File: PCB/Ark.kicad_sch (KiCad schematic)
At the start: 47 parts, among them P1 mode, P2 down, P3 up, SW1 EC12, SW2 EC12, SW3 EC12, SW4 EC12, SW5 EC12, SW6 EC12, SW7 EC12, SW8 EC12, U1 SeeeduinoXIAO, U2 ATmega328P-P, U3 ATmega328P-P, U4 74HC595

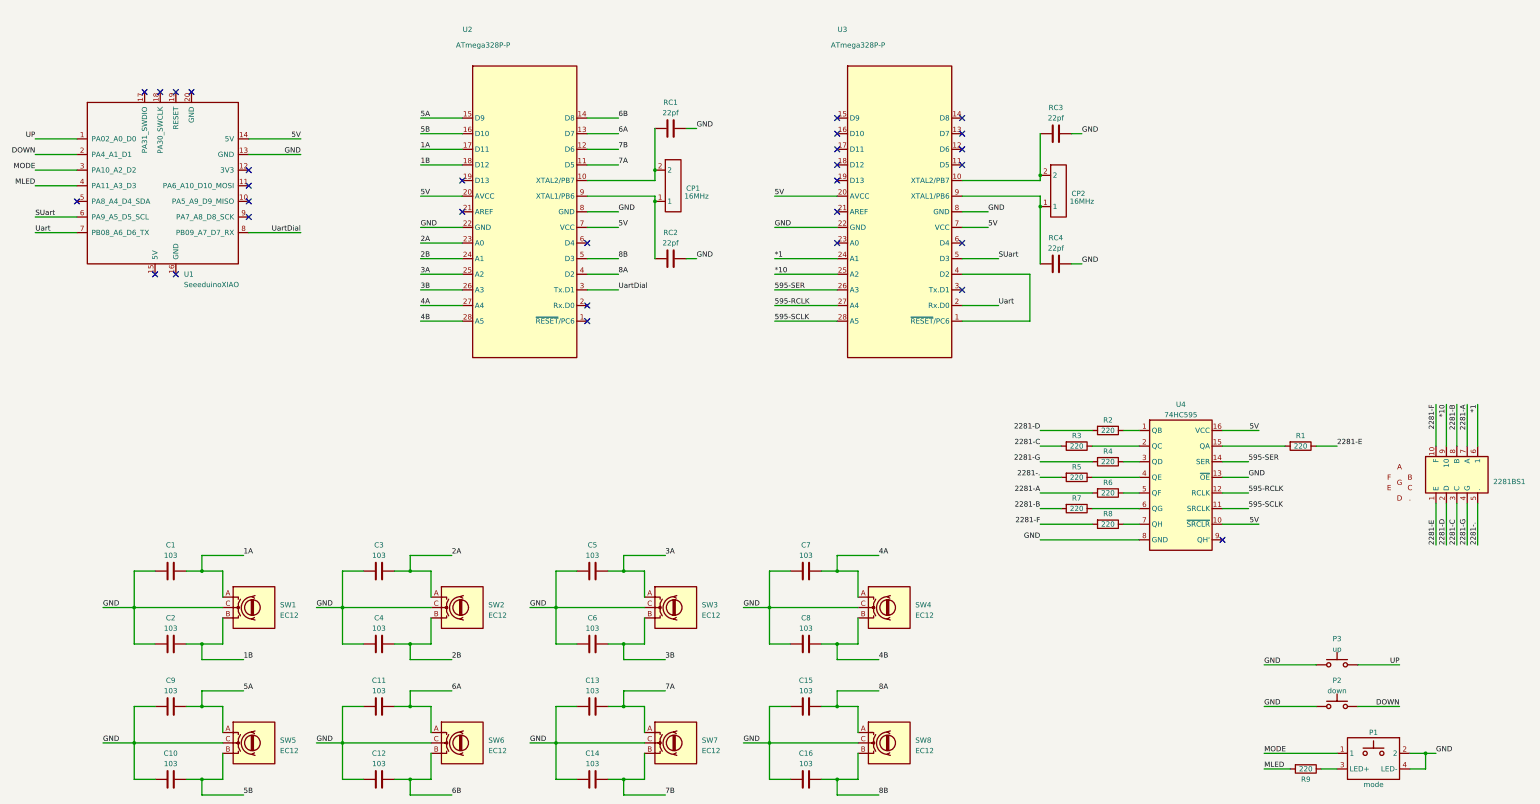
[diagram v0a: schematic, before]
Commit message: Add files via upload
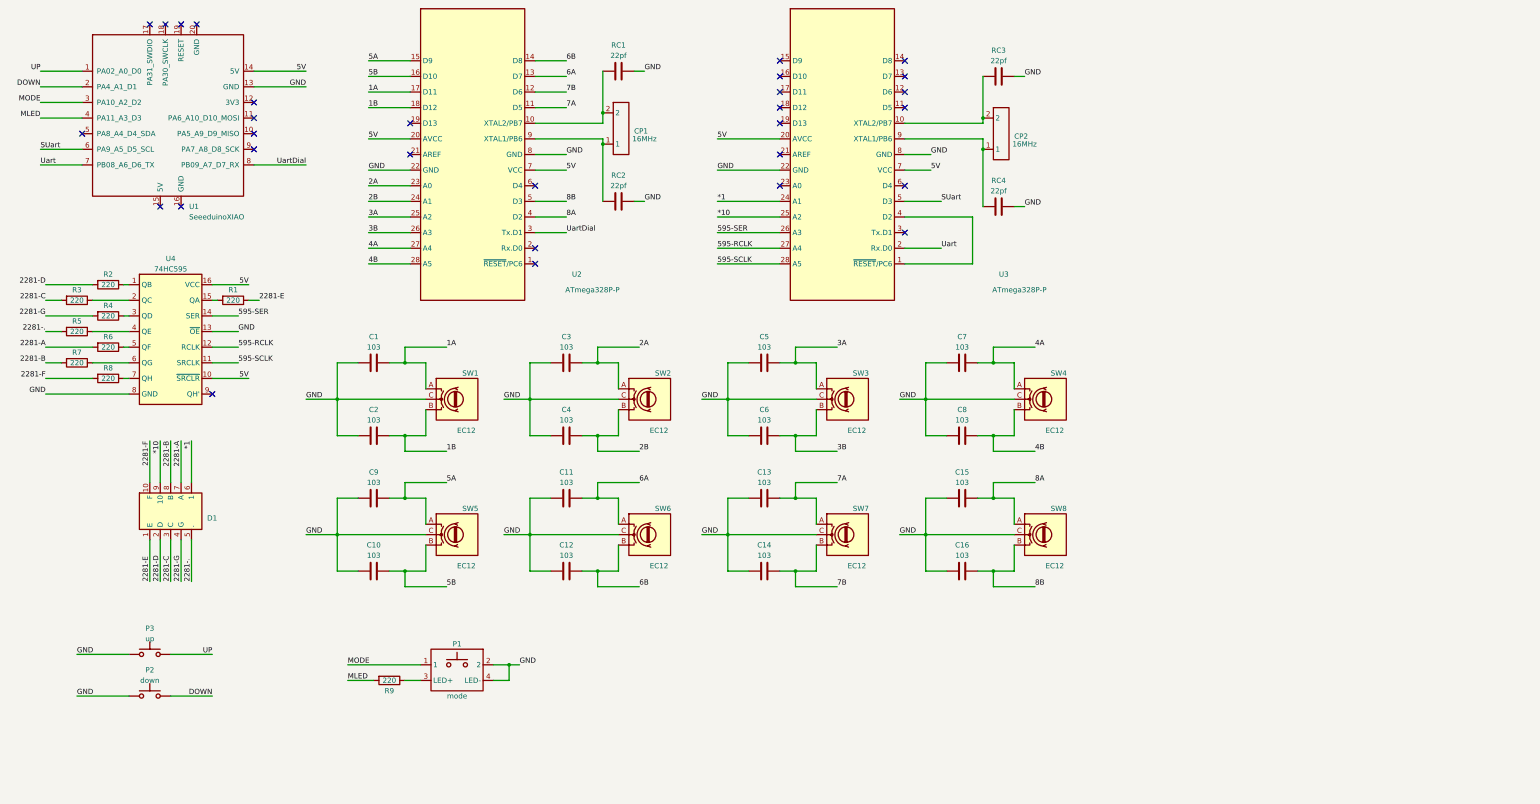
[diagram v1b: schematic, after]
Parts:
- D1: renamed from 2281BS1; symbol 2281BS:2281BS_7seg*2 -> 2281BS:2281
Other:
- title: Ark.*~ Product -> ark.*~
- moved on the sheet: C1, C10, C11, C12, C13, C14, C15, C16, C2, C3, C4, C5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
